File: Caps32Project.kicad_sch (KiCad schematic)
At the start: 31 parts, among them J1 Conn_01x08, J2 Sh 1.0, J3 Ph 2.0, J4 Conn_01x08, P1 USB_C_Plug_USB2.0, Q1 AO3401A, SW2 CK_KMS2xxGP, U1 IP5306

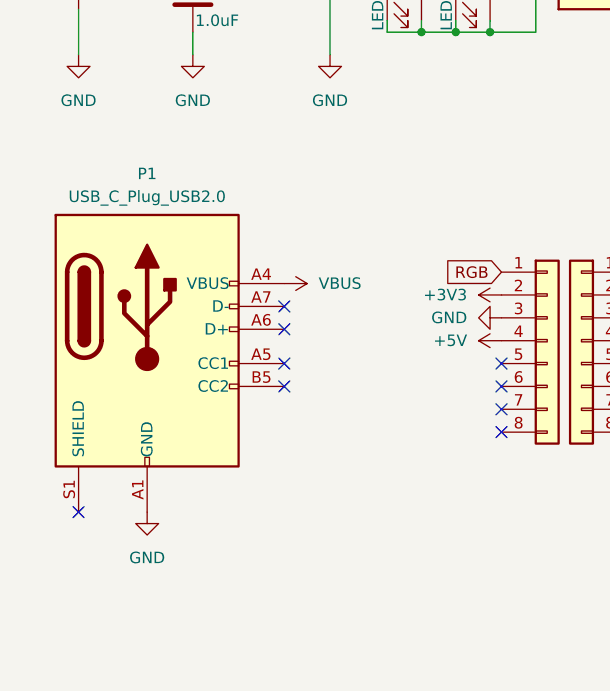
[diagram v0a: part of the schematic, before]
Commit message: Drop
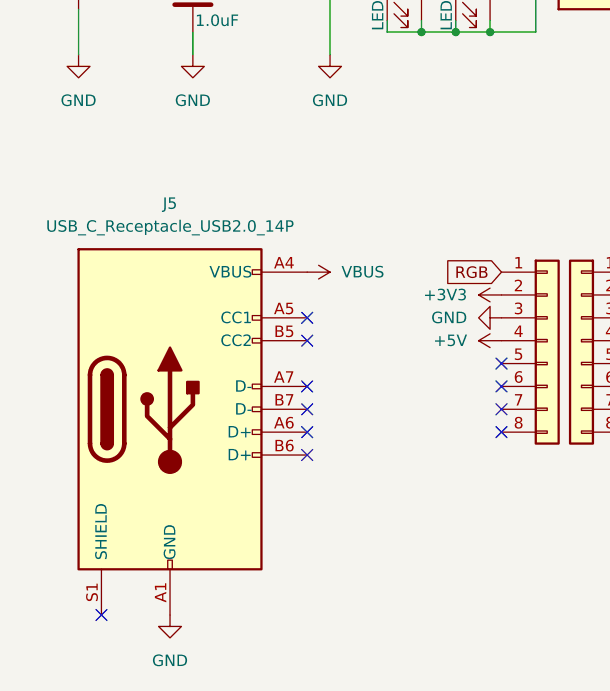
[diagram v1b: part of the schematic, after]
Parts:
- removed P1: USB_C_Plug_USB2.0, Connector_USB:USB_C_Receptacle_XKB_U262-16XN-4BVC11, symbol Connector:USB_C_Plug_USB2.0
- added J5: USB_C_Receptacle_USB2.0_14P, Connector_USB:USB_C_Receptacle_GCT_USB4105-xx-A_16P_TopMnt_Horizontal, symbol Connector:USB_C_Receptacle_USB2.0_14P
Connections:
- net GND: now also J5.A1 (GND), J5.A12 (GND), J5.B1 (GND), J5.B12 (GND)
- net VBUS: now also J5.A4 (VBUS), J5.A9 (VBUS), J5.B4 (VBUS), J5.B9 (VBUS)
- no-connect marks 16 -> 18
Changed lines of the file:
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@@
 	)
 	(no_connect
-		(at 45.72 77.47)
+		(at 48.26 88.9)
 	)
 	(no_connect
@@
 	)
 	(no_connect
-		(at 45.72 83.82)
+		(at 48.26 83.82)
 	)
 	(no_connect
@@
 	)
 	(no_connect
-		(at 45.72 81.28)
+		(at 48.26 91.44)
+	)
+	(no_connect
+		(at 48.26 76.2)
 	)
 	(no_connect
@@
 	)
 	(no_connect
-		(at 22.86 97.79)
+		(at 25.4 109.22)
 	)
 	(no_connect
@@
 	)
 	(no_connect
-		(at 45.72 74.93)
+		(at 48.26 78.74)
+	)
+	(no_connect
+		(at 48.26 86.36)
 	)
 	(no_connect
@@
 	)
 	(symbol
-		(lib_id "power:VBUS")
-		(at 45.72 72.39 270)
-		(unit 1)
-		(exclude_from_sim no)
-		(in_bom yes)
-		(on_board yes)
-		(dnp no)
-		(fields_autoplaced yes)
-		(property "Reference" "#PWR031"
-			(at 41.91 72.39 0)
-			(effects
-				(font
-					(size 1.27 1.27)
-				)
-				(hide yes)
-			)
-		)
-		(property "Value" "VBUS"
-			(at 49.53 72.3899 90)
-			(effects
-				(font
-					(size 1.27 1.27)
-				)
-				(justify left)
-			)
-		)
-		(property "Footprint" ""
-			(at 45.72 72.39 0)
-			(effects
-				(font
-					(size 1.27 1.27)
-				)
-				(hide yes)
-			)
-		)
-		(property "Datasheet" ""
-			(at 45.72 72.39 0)
-			(effects
-				(font
-					(size 1.27 1.27)
-				)
-				(hide yes)
-			)
-		)
-		(property "Description" "Power symbol creates a global label with name \"VBUS\""
-			(at 45.72 72.39 0)
-			(effects
-				(font
-					(size 1.27 1.27)
-				)
-				(hide yes)
-			)
-		)
-		(pin "1"
-		)
-		(instances
-			(project "Caps"
-				(path "/c1972a26-8b03-42e6-af88-e08ef9733d83"
-					(reference "#PWR031")
-					(unit 1)
-				)
-			)
-		)
-	)
-	(symbol
 		(lib_id "Switch:CK_KMS2xxGP")
 		(at 92.71 46.99 180)
@@
 	)
 	(symbol
+		(lib_id "power:VBUS")
+		(at 48.26 71.12 270)
+		(unit 1)
+		(exclude_from_sim no)
+		(in_bom yes)
+		(on_board yes)
+		(dnp no)
+		(fields_autoplaced yes)
+		(property "Reference" "#PWR021"
+			(at 44.45 71.12 0)
+			(effects
+				(font
+					(size 1.27 1.27)
+				)
+				(hide yes)
+			)
+		)
+		(property "Value" "VBUS"
+			(at 52.07 71.1199 90)
+			(effects
+				(font
+					(size 1.27 1.27)
+				)
+				(justify left)
+			)
+		)
+		(property "Footprint" ""
+			(at 48.26 71.12 0)
+			(effects
+				(font
+					(size 1.27 1.27)
+				)
+				(hide yes)
+			)
+		)
+		(property "Datasheet" ""
+			(at 48.26 71.12 0)
+			(effects
+				(font
+					(size 1.27 1.27)
+				)
+				(hide yes)
+			)
+		)
+		(property "Description" "Power symbol creates a global label with name \"VBUS\""
+			(at 48.26 71.12 0)
+			(effects
+				(font
+					(size 1.27 1.27)
+				)
+				(hide yes)
+			)
+		)
+		(pin "1"
+		)
+		(instances
+			(project "Caps32Project"
+				(path "/c1972a26-8b03-42e6-af88-e08ef9733d83"
+					(reference "#PWR021")
+					(unit 1)
+				)
+			)
+		)
+	)
+	(symbol
 		(lib_id "power:GND")
 		(at 83.82 88.9 90)
@@
 	(symbol
 		(lib_id "power:GND")
-		(at 30.48 97.79 0)
+		(at 33.02 109.22 0)
 		(unit 1)
 		(exclude_from_sim no)
@@
 		(fields_autoplaced yes)
 		(property "Reference" "#PWR027"
-			(at 30.48 104.14 0)
+			(at 33.02 115.57 0)
 			(effects
 				(font
@@
 		)
 		(property "Value" "GND"
-			(at 30.48 102.87 0)
+			(at 33.02 114.3 0)
 			(effects
 				(font
@@
 		)
 		(property "Footprint" ""
-			(at 30.48 97.79 0)
+			(at 33.02 109.22 0)
 			(effects
 				(font
@@
 		)
 		(property "Datasheet" ""
-			(at 30.48 97.79 0)
+			(at 33.02 109.22 0)
 			(effects
 				(font
@@
 		)
 		(property "Description" "Power symbol creates a global label with name \"GND\" , ground"
-			(at 30.48 97.79 0)
+			(at 33.02 109.22 0)
 			(effects
 				(font
@@
 	)
 	(symbol
+		(lib_id "Connector:USB_C_Receptacle_USB2.0_14P")
+		(at 33.02 86.36 0)
+		(unit 1)
+		(exclude_from_sim no)
+		(in_bom yes)
+		(on_board yes)
+		(dnp no)
+		(fields_autoplaced yes)
+		(property "Reference" "J5"
+			(at 33.02 63.5 0)
+			(effects
+				(font
+					(size 1.27 1.27)
+				)
+			)
+		)
+		(property "Value" "USB_C_Receptacle_USB2.0_14P"
+			(at 33.02 66.04 0)
+			(effects
+				(font
+					(size 1.27 1.27)
+				)
+			)
+		)
+		(property "Footprint" "Connector_USB:USB_C_Receptacle_GCT_USB4105-xx-A_16P_TopMnt_Horizontal"
+			(at 36.83 86.36 0)
+			(effects
+				(font
+					(size 1.27 1.27)
+				)
+				(hide yes)
+			)
+		)
+		(property "Datasheet" "https://www.usb.org/sites/default/files/documents/usb_type-c.zip"
+			(at 36.83 86.36 0)
+			(effects
+				(font
+					(size 1.27 1.27)
+				)
+				(hide yes)
+			)
+		)
+		(property "Description" "USB 2.0-only 14P Type-C Receptacle connector"
+			(at 33.02 86.36 0)
+			(effects
+				(font
+					(size 1.27 1.27)
+				)
+				(hide yes)
+			)
+		)
+		(pin "A12"
+		)
+		(pin "B9"
+		)
+		(pin "A1"
+		)
+		(pin "A4"
+		)
+		(pin "A6"
+		)
+		(pin "A9"
+		)
+		(pin "B4"
+		)
+		(pin "B6"
+		)
+		(pin "A5"
+		)
+		(pin "S1"
+		)
+		(pin "B7"
+		)
+		(pin "B12"
+		)
+		(pin "A7"
+		)
+		(pin "B1"
+		)
+		(pin "B5"
+		)
+		(instances
+			(project ""
+				(path "/c1972a26-8b03-42e6-af88-e08ef9733d83"
+					(reference "J5")
+					(unit 1)
+				)
+			)
+		)
+	)
+	(symbol
 		(lib_id "power:+5V")
 		(at 69.85 78.74 90)
@@
 					(unit 1)
 				)
-			)
-		)
-	)
-	(symbol
-		(lib_id "Connector:USB_C_Plug_USB2.0")
-		(at 30.48 74.93 0)
-		(unit 1)
-		(exclude_from_sim no)
-		(in_bom yes)
-		(on_board yes)
-		(dnp no)
-		(fields_autoplaced yes)
-		(property "Reference" "P1"
-			(at 30.48 60.198 0)
-			(effects
-				(font
-					(size 1.27 1.27)
-				)
-			)
-		)
-		(property "Value" "USB_C_Plug_USB2.0"
-			(at 30.48 62.738 0)
-			(effects
-				(font
-					(size 1.27 1.27)
-				)
-			)
-		)
-		(property "Footprint" "Connector_USB:USB_C_Receptacle_XKB_U262-16XN-4BVC11"
-			(at 34.29 74.93 0)
-			(effects
-				(font
-					(size 1.27 1.27)
-				)
-				(hide yes)
-			)
-		)
-		(property "Datasheet" "https://www.usb.org/sites/default/files/documents/usb_type-c.zip"
-			(at 34.29 74.93 0)
-			(effects
-				(font
-					(size 1.27 1.27)
-				)
-				(hide yes)
-			)
-		)
-		(property "Description" "USB 2.0-only Type-C Plug connector"
-			(at 30.48 74.93 0)
-			(effects
-				(font
-					(size 1.27 1.27)
-				)
-				(hide yes)
-			)
-		)
-		(pin "B12"
-		)
-		(pin "A1"
-		)
-		(pin "S1"
-		)
-		(pin "A4"
-		)
-		(pin "A12"
-		)
-		(pin "A7"
-		)
-		(pin "A5"
-		)
-		(pin "B1"
-		)
-		(pin "A9"
-		)
-		(pin "B5"
-		)
-		(pin "A6"
-		)
-		(pin "B9"
-		)
-		(pin "B4"
-		)
-		(instances
-			(project ""
-				(path "/c1972a26-8b03-42e6-af88-e08ef9733d83"
-					(reference "P1")
-					(unit 1)
-				)

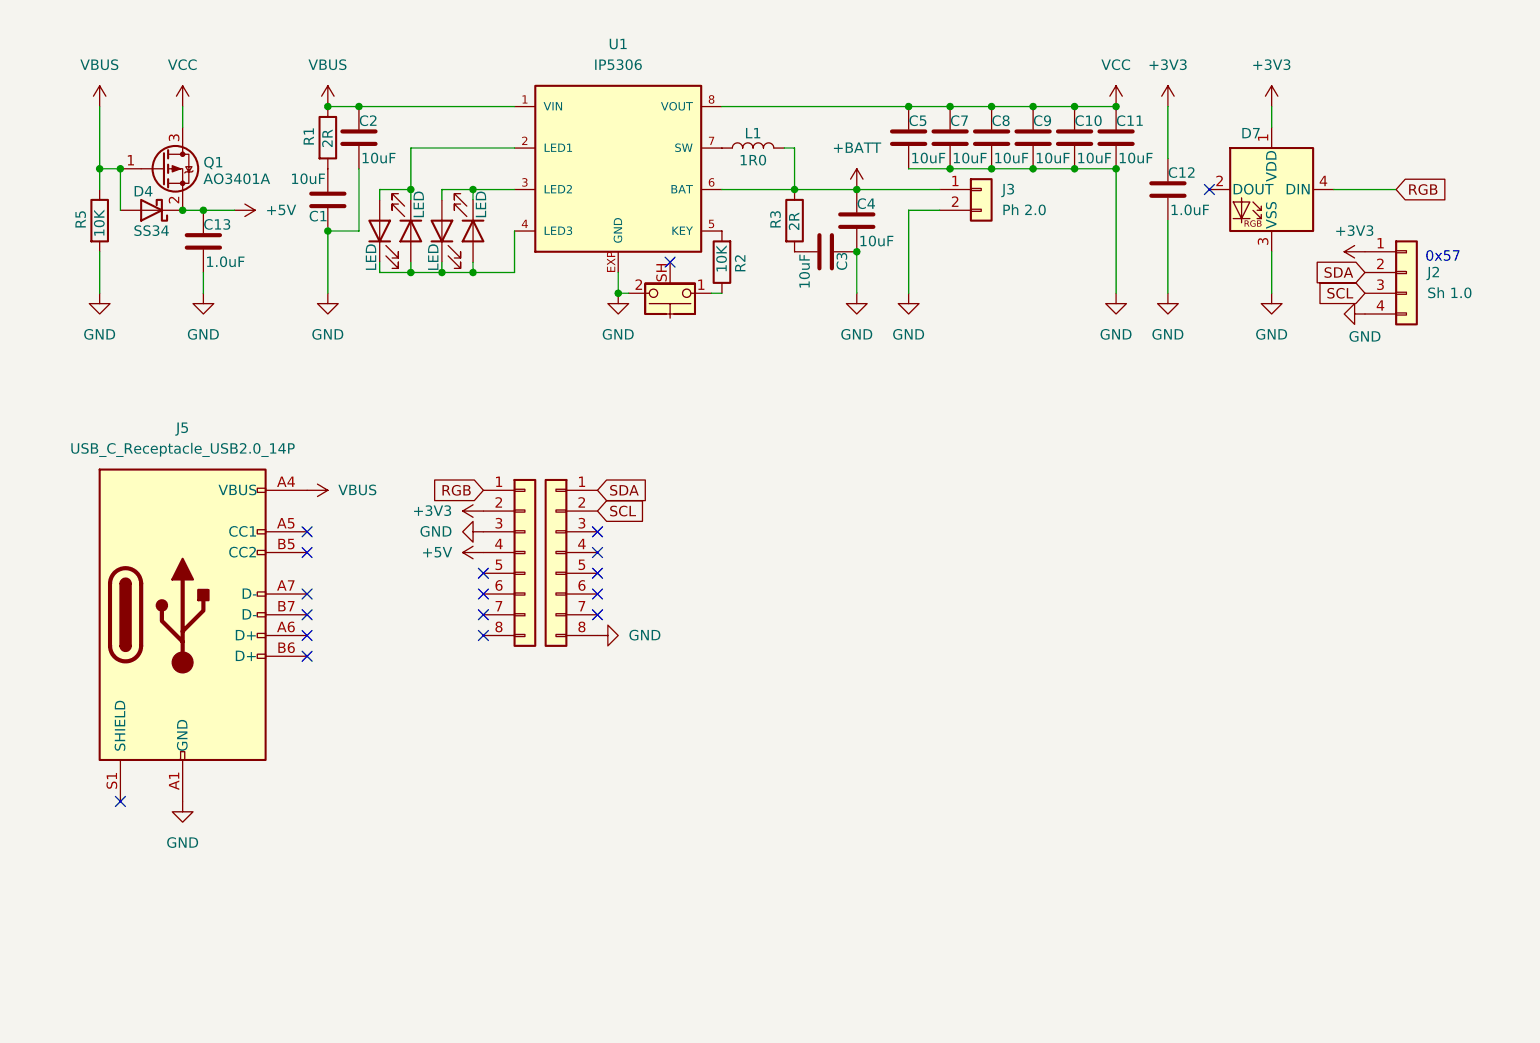
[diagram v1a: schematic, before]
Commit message: Update Board
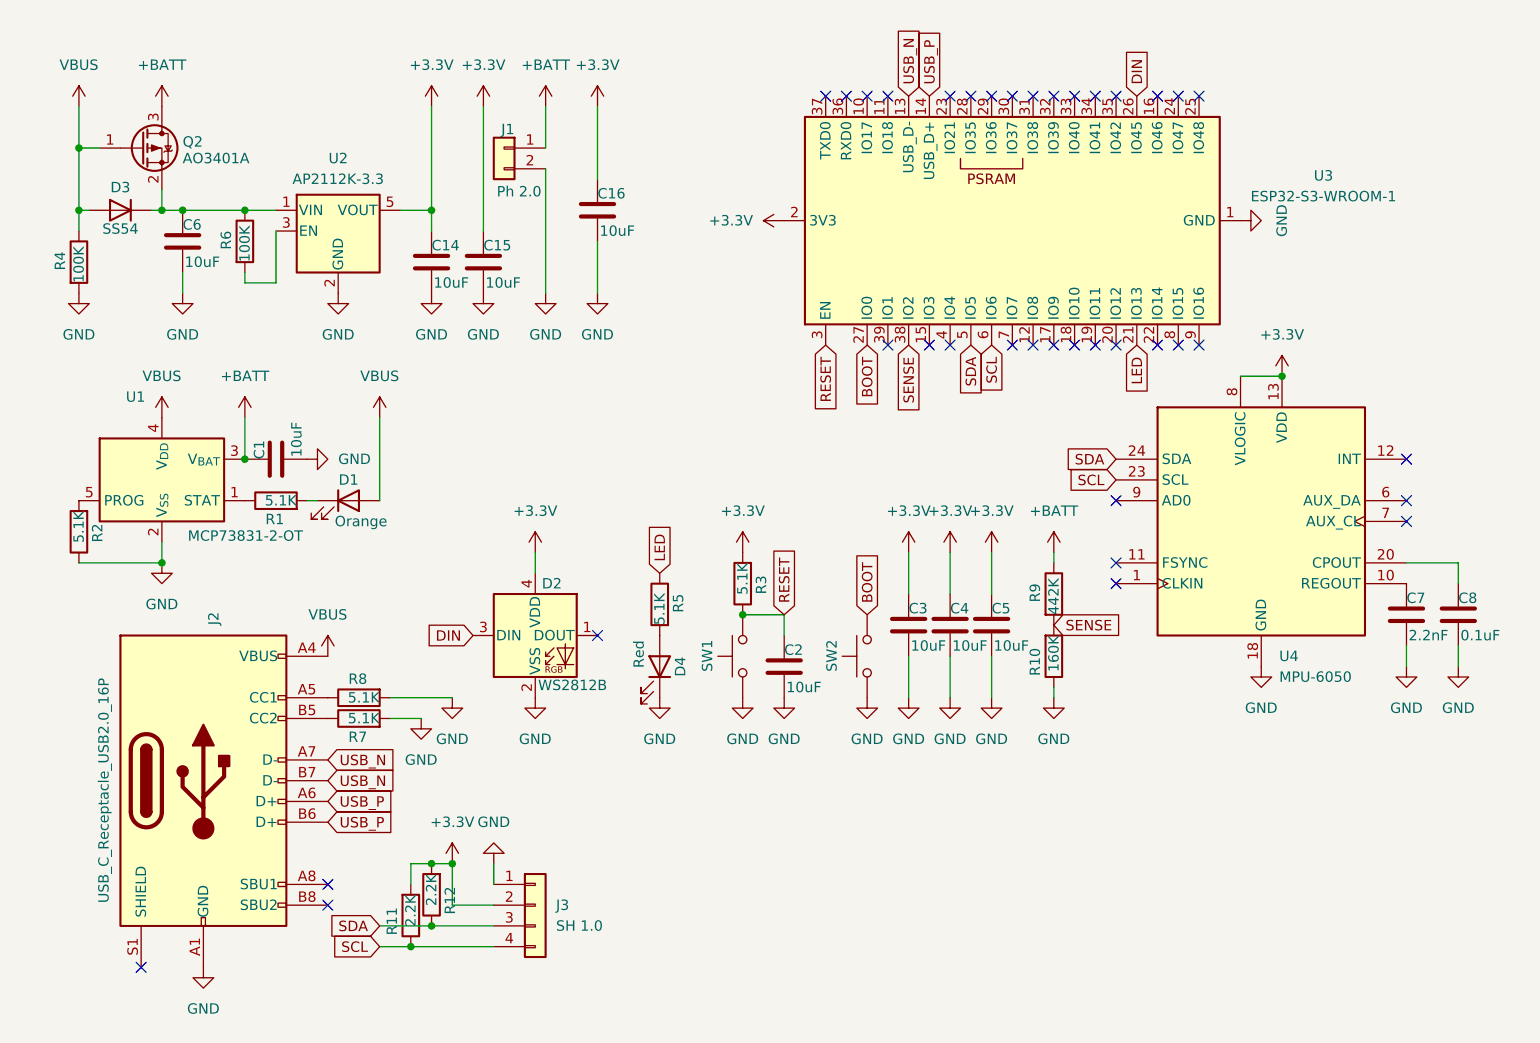
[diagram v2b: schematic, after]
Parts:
- removed C10, C11, C9: 10uF, Capacitor_SMD:C_0402_1005Metric_Pad0.74x0.62mm_HandSolder, symbol Device:C
- removed C12, C13: 1.0uF, Capacitor_SMD:C_0402_1005Metric_Pad0.74x0.62mm_HandSolder, symbol Device:C
- removed D2, D5, D6: LED, LED_SMD:LED_0402_1005Metric_Pad0.77x0.64mm_HandSolder, symbol Device:LED
- removed D4: SS34, Diode_SMD:D_SMA, symbol Diode:SS34
- removed D7: WS2812B, LED_SMD:LED_WS2812B_PLCC4_5.0x5.0mm_P3.2mm, symbol LED:WS2812B
- removed J1, J4: Conn_01x08, Connector_PinHeader_2.54mm:PinHeader_1x08_P2.54mm_Vertical, symbol Connector_Generic:Conn_01x08
- removed J2: Sh 1.0, Connector_JST:JST_SH_SM04B-SRSS-TB_1x04-1MP_P1.00mm_Horizontal, symbol Connector_Generic:Conn_01x04
- removed J3: Ph 2.0, Connector_JST:JST_PH_S2B-PH-K_1x02_P2.00mm_Horizontal, symbol Connector_Generic:Conn_01x02
- removed J5: USB_C_Receptacle_USB2.0_14P, Connector_USB:USB_C_Receptacle_GCT_USB4105-xx-A_16P_TopMnt_Horizontal, symbol Connector:USB_C_Receptacle_USB2.0_14P
- removed L1: 1R0, Inductor_SMD:L_6.3x6.3_H3, symbol Device:L
- removed Q1: AO3401A, Package_TO_SOT_SMD:SOT-23, symbol Transistor_FET:AO3401A
- removed SW2: CK_KMS2xxGP, Button_Switch_SMD:SW_SPST_CK_KMS2xxGP, symbol Switch:CK_KMS2xxGP
- removed U1: IP5306, Custom:IP5306, symbol Custom:IP5306
- added C14, C15, C16, C6: 10uF, Capacitor_SMD:C_0402_1005Metric, symbol Device:C
- added D2: WS2812B, LED_SMD:LED_WS2812B-2020_PLCC4_2.0x2.0mm, symbol LED:WS2812B-2020
- added D3: SS54, Diode_SMD:D_SMA, symbol Device:D
- added D4: Red, LED_SMD:LED_0402_1005Metric, symbol Device:LED
- added J1: Ph 2.0, Connector_JST:JST_PH_S2B-PH-SM4-TB_1x02-1MP_P2.00mm_Horizontal, symbol Connector_Generic:Conn_01x02
- added J2: USB_C_Receptacle_USB2.0_16P, Connector_USB:USB_C_Receptacle_GCT_USB4105-xx-A_16P_TopMnt_Horizontal, symbol Connector:USB_C_Receptacle_USB2.0_16P
- added J3: SH 1.0, Connector_JST:JST_SH_BM04B-SRSS-TB_1x04-1MP_P1.00mm_Vertical, symbol Connector_Generic:Conn_01x04
- added Q2: AO3401A, Package_TO_SOT_SMD:SOT-23, symbol Transistor_FET:AO3401A
- added R10: 160K, Resistor_SMD:R_0805_2012Metric, symbol Device:R
- added R11, R12: 2.2K, Resistor_SMD:R_0402_1005Metric, symbol Device:R
- added R4, R6: 100K, Resistor_SMD:R_0201_0603Metric, symbol Device:R
- added R7, R8: 5.1K, Resistor_SMD:R_0402_1005Metric, symbol Device:R
- added R9: 442K, Resistor_SMD:R_0805_2012Metric, symbol Device:R
- added SW1, SW2: SW_Push, Button_Switch_SMD:SW_Push_SPST_NO_Alps_SKRK, symbol Switch:SW_Push
- added U1: MCP73831-2-OT, Package_TO_SOT_SMD:SOT-23-5, symbol Battery_Management:MCP73831-2-OT
- added U2: AP2112K-3.3, Package_TO_SOT_SMD:SOT-23-5, symbol Regulator_Linear:AP2112K-3.3
- added U3: ESP32-S3-WROOM-1, RF_Module:ESP32-S3-WROOM-1, symbol RF_Module:ESP32-S3-WROOM-1
- added U4: MPU-6050, Sensor_Motion:InvenSense_QFN-24_4x4mm_P0.5mm, symbol Sensor_Motion:MPU-6050
- C1, C2, C3, C4, C5: footprint Capacitor_SMD:C_0402_1005Metric_Pad0.74x0.62mm_HandSolder -> Capacitor_SMD:C_0402_1005Metric
- C7: value 10uF -> 2.2nF; footprint Capacitor_SMD:C_0402_1005Metric_Pad0.74x0.62mm_HandSolder -> Capacitor_SMD:C_0603_1608Metric
- C8: value 10uF -> 0.1uF; footprint Capacitor_SMD:C_0402_1005Metric_Pad0.74x0.62mm_HandSolder -> Capacitor_SMD:C_0201_0603Metric
- D1: value LED -> Orange; footprint LED_SMD:LED_0402_1005Metric_Pad0.77x0.64mm_HandSolder -> LED_SMD:LED_0402_1005Metric
- R1, R3: value 2R -> 5.1K; footprint Resistor_SMD:R_0402_1005Metric_Pad0.72x0.64mm_HandSolder -> Resistor_SMD:R_0402_1005Metric
- R2, R5: value 10K -> 5.1K; footprint Resistor_SMD:R_0402_1005Metric_Pad0.72x0.64mm_HandSolder -> Resistor_SMD:R_0402_1005Metric
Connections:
- net +BATT: now also C1.1, J1.1 (Pin_1), Q2.3 (D), R9.1, U1.3 (V_{BAT}); no longer C4.1, R3.1
- net GND: now also C1.2, C3.2, R2.1, C14.2, C15.2, C16.2, C6.2, D2.2 (VSS), D4.1 (K), J1.2 (Pin_2), J2.A1 (GND), J2.A12 (GND), J2.B1 (GND), J2.B12 (GND), J3.1 (Pin_1), R10.1, R4.2, R7.2, R8.2, SW1.1, SW2.1, U1.2 (V_{SS}), U2.2 (GND), U3.1 (GND), U3.40 (GND), U3.41 (GND), U4.18 (GND); no longer C1.1, C3.1, R5.2
- net SCL: now also J3.4 (Pin_4), R11.1, U3.6 (IO6), U4.23 (SCL)
- net SDA: now also J3.3 (Pin_3), R12.1, U3.5 (IO5), U4.24 (SDA)
- net VBUS: now also D1.2 (A), D3.2 (A), J2.A4 (VBUS), J2.A9 (VBUS), J2.B4 (VBUS), J2.B9 (VBUS), Q2.1 (G), R4.1, U1.4 (V_{DD}); no longer C2.1, R1.1, R5.1
- net at D1.1 (K): now also R1.2
- net at R2.2: now also U1.5 (PROG)
- net +3.3V: now reaches R3.2
- net +3.3V: now also C3.1, C4.1, C5.1, C14.1, C15.1, C16.1, D2.4 (VDD), J3.2 (Pin_2), R11.2, R12.2, U2.5 (VOUT), U3.2 (3V3), U4.13 (VDD), U4.8 (VLOGIC); no longer C3.2
- removed net VCC: C5.1, C7.1, C8.1
- new net: J2.B5 (CC2), R7.1
- new net: C7.1, U4.10 (REGOUT)
- new net: R1.1, U1.1 (STAT)
- new net: C8.1, U4.20 (CPOUT)
- new net: J2.A5 (CC1), R8.1
- new net: C6.1, D3.1 (K), Q2.2 (S), R6.1, U2.1 (VIN)
- new net: R6.2, U2.3 (EN)
- new net: D4.2 (A), R5.2
- new net BOOT: SW2.2, U3.27 (IO0)
- new net DIN: D2.3 (DIN), U3.26 (IO45)
- new net LED: R5.1, U3.21 (IO13)
- new net RESET: C2.1, R3.1, SW1.2, U3.3 (EN)
- new net SENSE: R10.2, R9.2, U3.38 (IO2)
- new net USB_N: J2.A7 (D-), J2.B7 (D-), U3.13 (USB_D-)
- new net USB_P: J2.A6 (D+), J2.B6 (D+), U3.14 (USB_D+)
- no-connect marks 18 -> 38
